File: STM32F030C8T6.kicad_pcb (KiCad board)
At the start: 2 copper layers, 25.4 x 55.9 mm, 29 parts, among them SW1 SW_Push, SW2 SW_Push, U1 STM32F030C8T6, U2 AMS1117-3.3

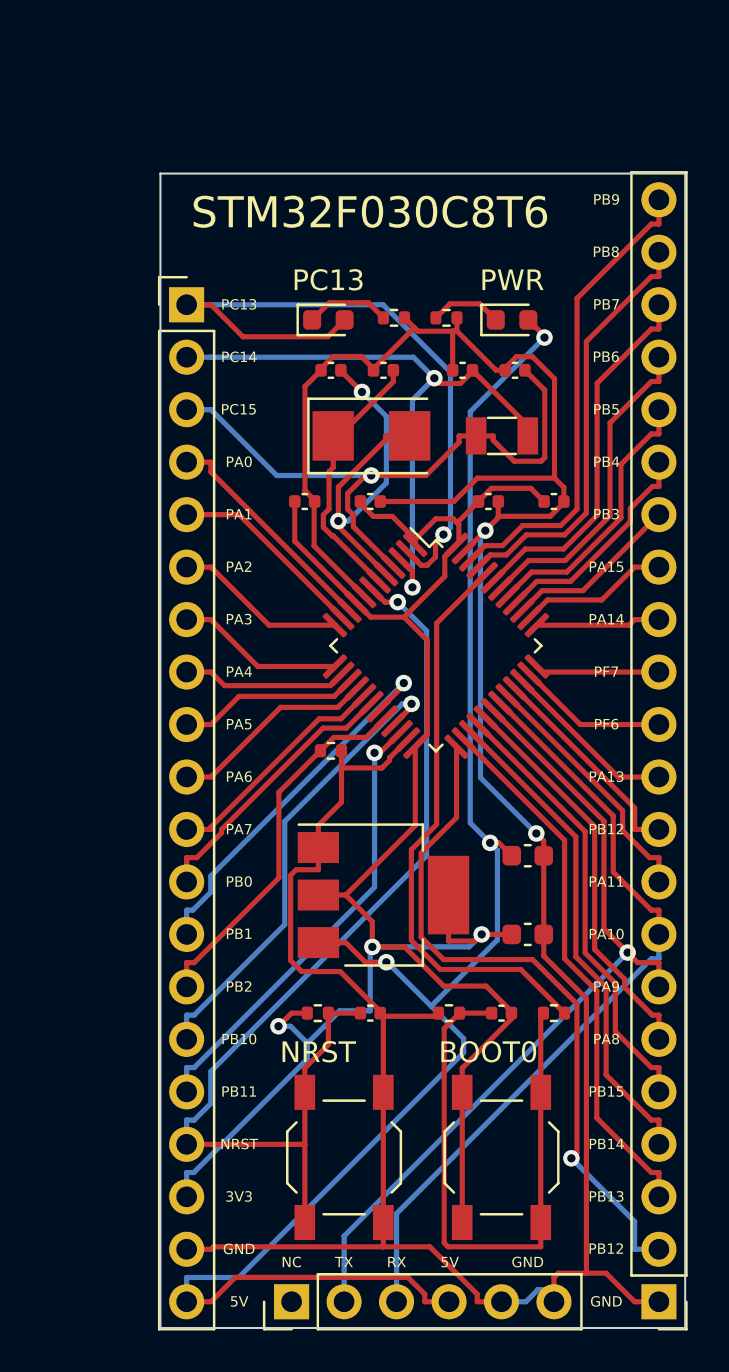
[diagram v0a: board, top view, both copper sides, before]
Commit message: Add files via upload
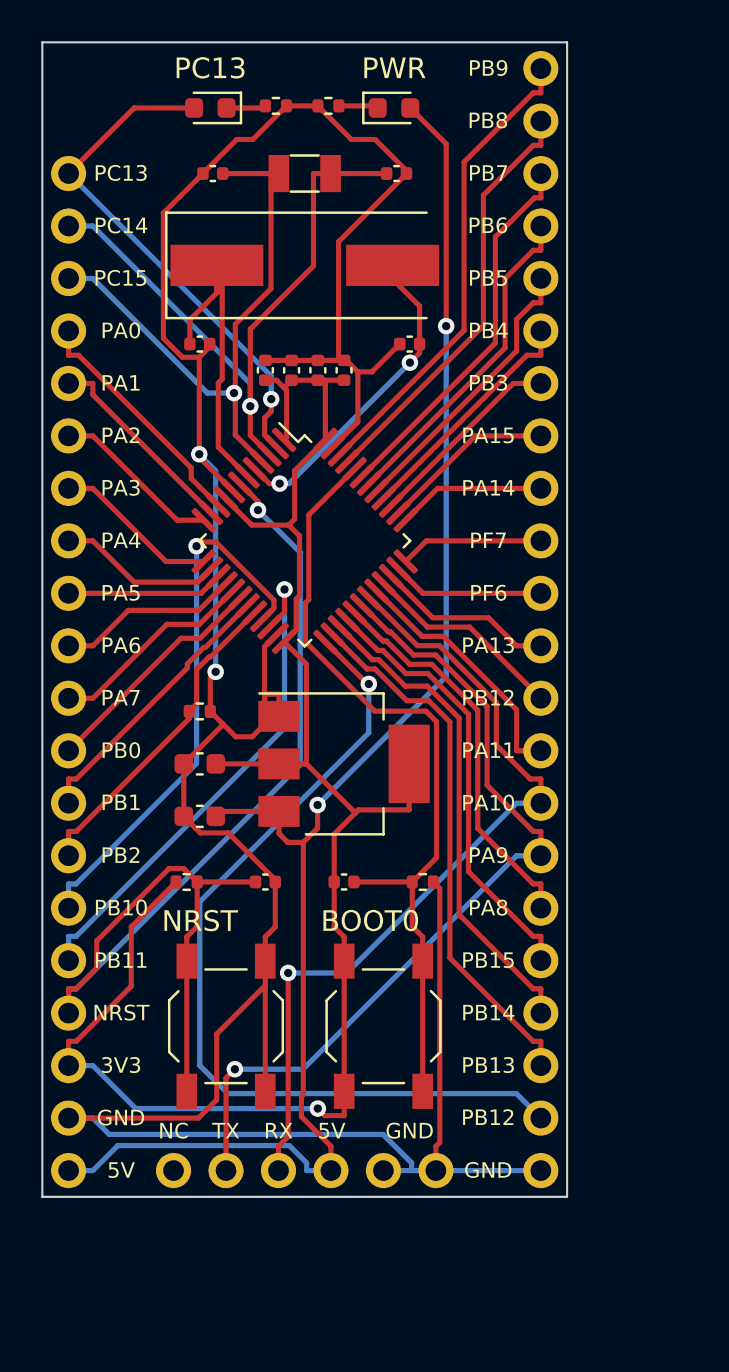
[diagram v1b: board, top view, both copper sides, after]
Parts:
- removed R6: 100KΩ, Resistor_SMD:R_0402_1005Metric
- R2: value 100KΩ -> 10KΩ
- R3: value 1KΩ -> 10KΩ
- XTAL2: footprint Crystal:Crystal_SMD_5032-2Pin_5.0x3.2mm -> Crystal:Crystal_SMD_HC49-SD
- moved R3 18.9 mm to (134.0, 111.8), turned to 180 degrees
- moved C12 17.9 mm to (134.6, 106.0), turned to 180 degrees
- moved C2 17.5 mm to (135.3, 77.5)
- moved C11 16.0 mm to (134.6, 108.6), turned to 180 degrees
- moved XTAL1 15.9 mm to (139.7, 77.5)
- moved C10 13.1 mm to (140.3, 87.0), turned to 90 degrees
- moved D1 11.7 mm to (135.1, 74.3), turned to 180 degrees
- moved D2 11.7 mm to (144.0, 74.3)
- moved R4 11.7 mm to (138.3, 74.2)
- moved R5 11.7 mm to (140.8, 74.2), turned to 180 degrees
- moved C1 10.0 mm to (144.1, 77.5), turned to 180 degrees
- moved C5 9.92 mm to (141.6, 111.8), turned to 180 degrees
- moved C9 9.44 mm to (141.6, 87.0), turned to 90 degrees
- moved C4 8.98 mm to (134.6, 85.7), turned to 180 degrees
- moved XTAL2 8.86 mm to (139.7, 81.9)
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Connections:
- C5 pad 1: Net-(C5-Pad1) -> BOOT0
- R2 pad 1: GND -> BOOT0
- R2 pad 2: Net-(C5-Pad1) -> GND
- R3 pad 1: Net-(C5-Pad1) -> NRST
- R3 pad 2: BOOT0 -> +3.3V
- SW2 pad 2: Net-(C5-Pad1) -> BOOT0
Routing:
- net Net-(C5-Pad1): track 29.1 -> 0.00 mm
- net +3.3V: track 96.3 -> 84.1 mm, vias 3 -> 1
- net BOOT0: track 28.1 -> 38.7 mm
- net PB12: track 33.2 -> 42.4 mm
- net PC13: track 33.8 -> 25.1 mm
- net +5V: track 80.8 -> 75.2 mm, vias 3 -> 2
- net PB1: track 18.5 -> 13.4 mm, vias 1 -> 0
- net NRST: track 51.3 -> 55.7 mm
- net PF1: track 13.0 -> 17.1 mm
- net PB10: track 22.6 -> 26.5 mm
- net PF0: track 19.2 -> 15.7 mm
- net PC15: track 30.9 -> 28.3 mm
- net PB11: track 22.1 -> 24.6 mm
- net PB2: track 18.2 -> 15.8 mm
- net Net-(D1-Pad1): track 4.10 -> 1.92 mm
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
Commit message: Add files via upload
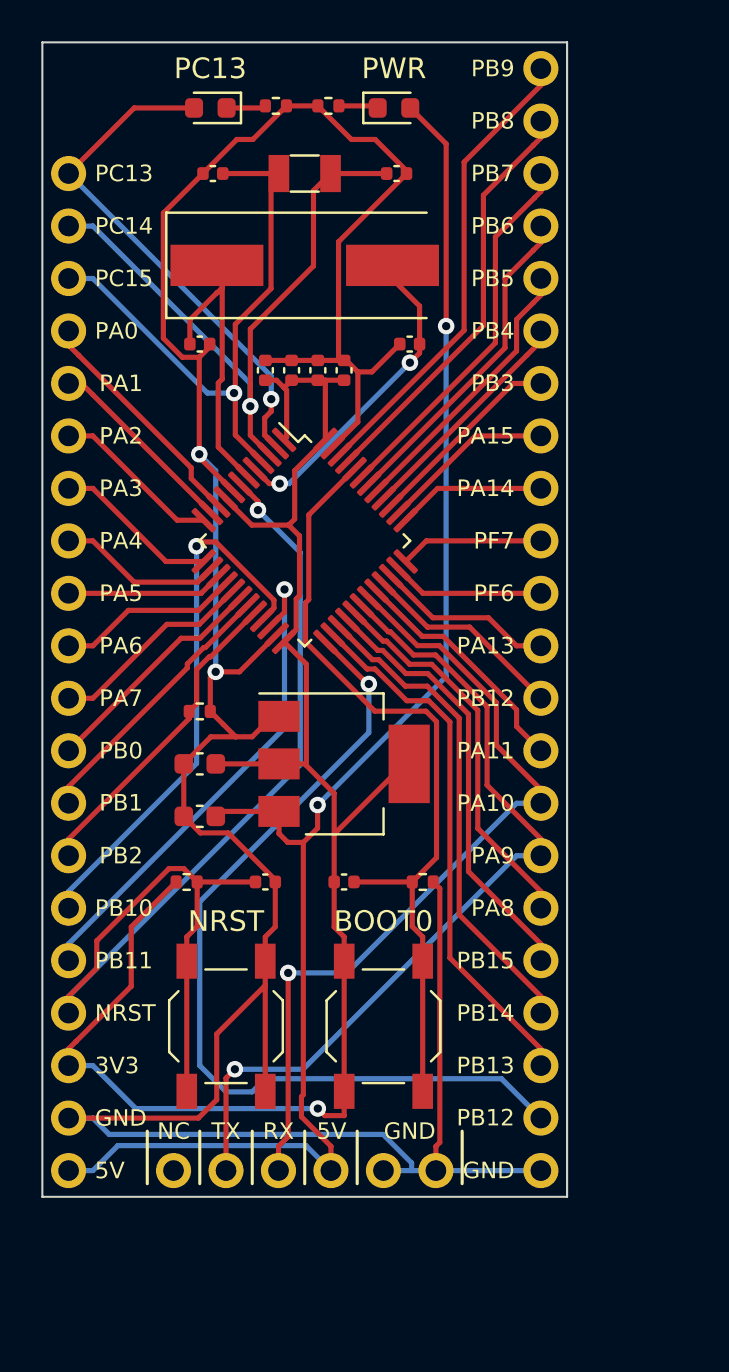
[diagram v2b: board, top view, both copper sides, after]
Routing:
- net GND: track 151.1 -> 148.8 mm
- net PF1: track 17.1 -> 14.8 mm
- net +3.3V: track 84.1 -> 83.2 mm
- net PA11: track 12.3 -> 11.6 mm
- net PB12: track 42.4 -> 42.9 mm
